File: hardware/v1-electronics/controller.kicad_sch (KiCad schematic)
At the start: 35 parts, among them IC1 IS31FL3733-QFLS4-TR, IC2 IS31FL3733-QFLS4-TR, J2 Conn_01x03, U1 MDBT50Q-1MV2

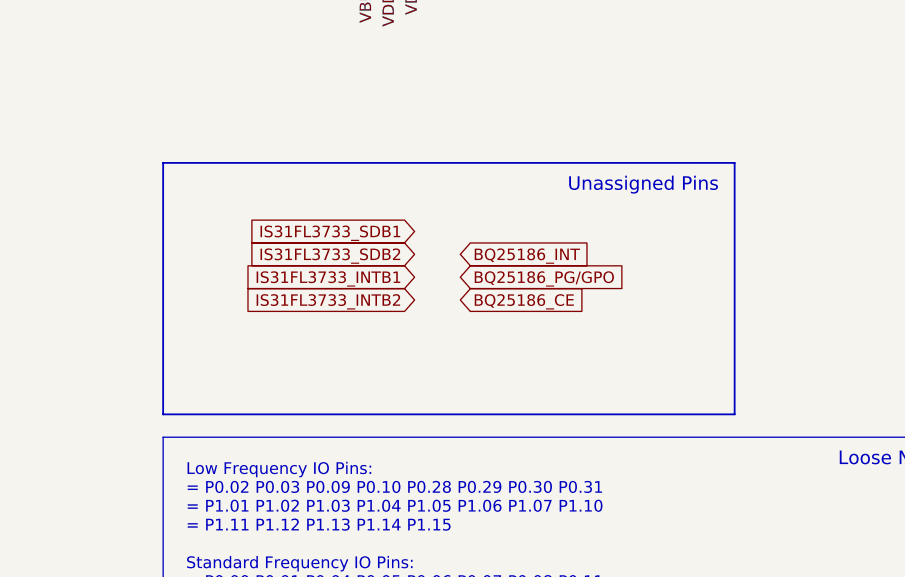
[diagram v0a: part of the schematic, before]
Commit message: refactor(v1 hardware): power system
Beefed up power system.
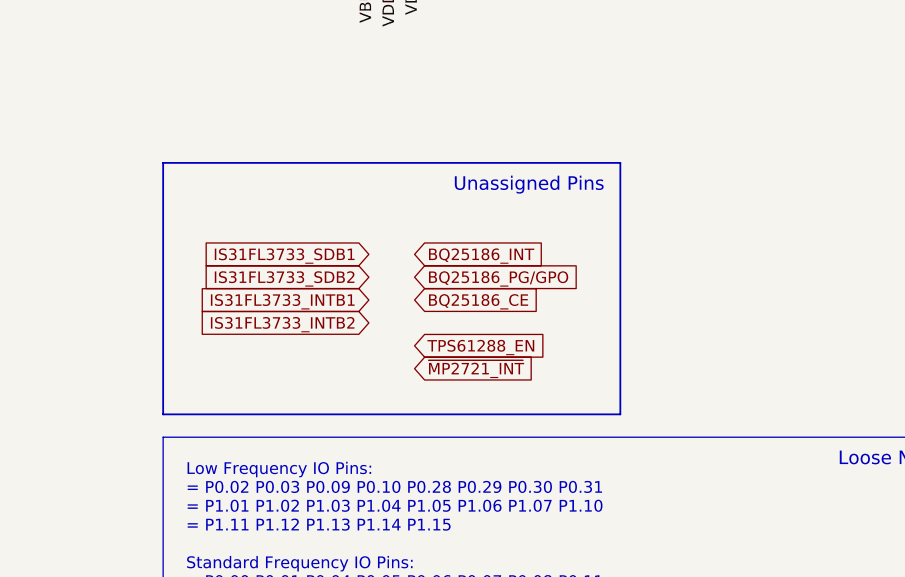
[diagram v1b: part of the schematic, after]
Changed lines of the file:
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@@
 		)
 		(fill
-			(type none)
+			(type color)
+			(color 255 229 191 1)
 		)
 	)
@@
 	(rectangle
 		(start 317.5 149.86)
-		(end 381 177.8)
+		(end 368.3 177.8)
 		(stroke
 			(width 0.2)
@@
 	(text "Unassigned Pins"
 		(exclude_from_sim no)
-		(at 370.84 152.4 0)
+		(at 358.14 152.4 0)
 		(effects
 			(font
@@
 		)
 	)
+	(global_label "TPS61288_EN"
+		(shape input)
+		(at 345.44 170.18 0)
+		(fields_autoplaced yes)
+		(effects
+			(font
+				(size 1.27 1.27)
+			)
+			(justify left)
+		)
+		(property "Intersheetrefs" "${INTERSHEET_REFS}"
+			(at 361.3669 170.18 0)
+			(hide yes)
+			(show_name no)
+			(do_not_autoplace no)
+			(effects
+				(font
+					(size 1.27 1.27)
+				)
+				(justify left)
+			)
+		)
+	)
 	(global_label "CS4_2"
 		(shape input)
@@
 	(global_label "BQ25186_INT"
 		(shape input)
-		(at 350.52 160.02 0)
+		(at 345.44 160.02 0)
 		(fields_autoplaced yes)
 		(effects
@@
 		)
 		(property "Intersheetrefs" "${INTERSHEET_REFS}"
-			(at 366.0237 160.02 0)
+			(at 360.9437 160.02 0)
 			(hide yes)
 			(show_name no)
@@
 	(global_label "IS31FL3733_INTB2"
 		(shape input)
-		(at 345.44 165.1 180)
+		(at 340.36 167.64 180)
 		(fields_autoplaced yes)
 		(effects
@@
 		)
 		(property "Intersheetrefs" "${INTERSHEET_REFS}"
-			(at 337.0724 165.1 0)
+			(at 331.9924 167.64 0)
 			(hide yes)
 			(show_name no)
@@
 	(global_label "BQ25186_PG{slash}GPO"
 		(shape input)
-		(at 350.52 162.56 0)
+		(at 345.44 162.56 0)
 		(fields_autoplaced yes)
 		(effects
@@
 		)
 		(property "Intersheetrefs" "${INTERSHEET_REFS}"
-			(at 370.8618 162.56 0)
+			(at 365.7818 162.56 0)
 			(hide yes)
 			(show_name no)
@@
 		)
 	)
+	(global_label "~{MP2721_INT}"
+		(shape input)
+		(at 345.44 172.72 0)
+		(fields_autoplaced yes)
+		(effects
+			(font
+				(size 1.27 1.27)
+			)
+			(justify left)
+		)
+		(property "Intersheetrefs" "${INTERSHEET_REFS}"
+			(at 359.8551 172.72 0)
+			(hide yes)
+			(show_name no)
+			(do_not_autoplace no)
+			(effects
+				(font
+					(size 1.27 1.27)
+				)
+				(justify left)
+			)
+		)
+	)
 	(global_label "RE10_B-Channel"
 		(shape input)
@@
 	(global_label "BQ25186_CE"
 		(shape input)
-		(at 350.52 165.1 0)
+		(at 345.44 165.1 0)
 		(fields_autoplaced yes)
 		(effects
@@
 		)
 		(property "Intersheetrefs" "${INTERSHEET_REFS}"
-			(at 365.5398 165.1 0)
+			(at 360.4598 165.1 0)
 			(hide yes)
 			(show_name no)
@@
 	(global_label "IS31FL3733_INTB1"
 		(shape input)
-		(at 345.44 162.56 180)
+		(at 340.36 165.1 180)
 		(fields_autoplaced yes)
 		(effects
@@
 		)
 		(property "Intersheetrefs" "${INTERSHEET_REFS}"
-			(at 337.0724 162.56 0)
+			(at 331.9924 165.1 0)
 			(hide yes)
 			(show_name no)
@@
 	(global_label "IS31FL3733_SDB2"
 		(shape input)
-		(at 345.44 160.02 180)
+		(at 340.36 162.56 180)
 		(fields_autoplaced yes)
 		(effects
@@
 		)
 		(property "Intersheetrefs" "${INTERSHEET_REFS}"
-			(at 337.4958 160.02 0)
+			(at 332.4158 162.56 0)
 			(hide yes)
 			(show_name no)
@@
 	(global_label "IS31FL3733_SDB1"
 		(shape input)
-		(at 345.44 157.48 180)
+		(at 340.36 160.02 180)
 		(fields_autoplaced yes)
 		(effects
@@
 		)
 		(property "Intersheetrefs" "${INTERSHEET_REFS}"
-			(at 337.4958 157.48 0)
+			(at 332.4158 160.02 0)
 			(hide yes)
 			(show_name no)
